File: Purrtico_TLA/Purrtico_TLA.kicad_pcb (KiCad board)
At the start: 2 copper layers, 100 x 50 mm, 67 parts, among them J1 XLR3, J3 Conn_01x02, J4 XLR3, J5 Conn_01x02, J7 Conn_02x05_Odd_Even, U1 OPA1679, U2 OPA1679

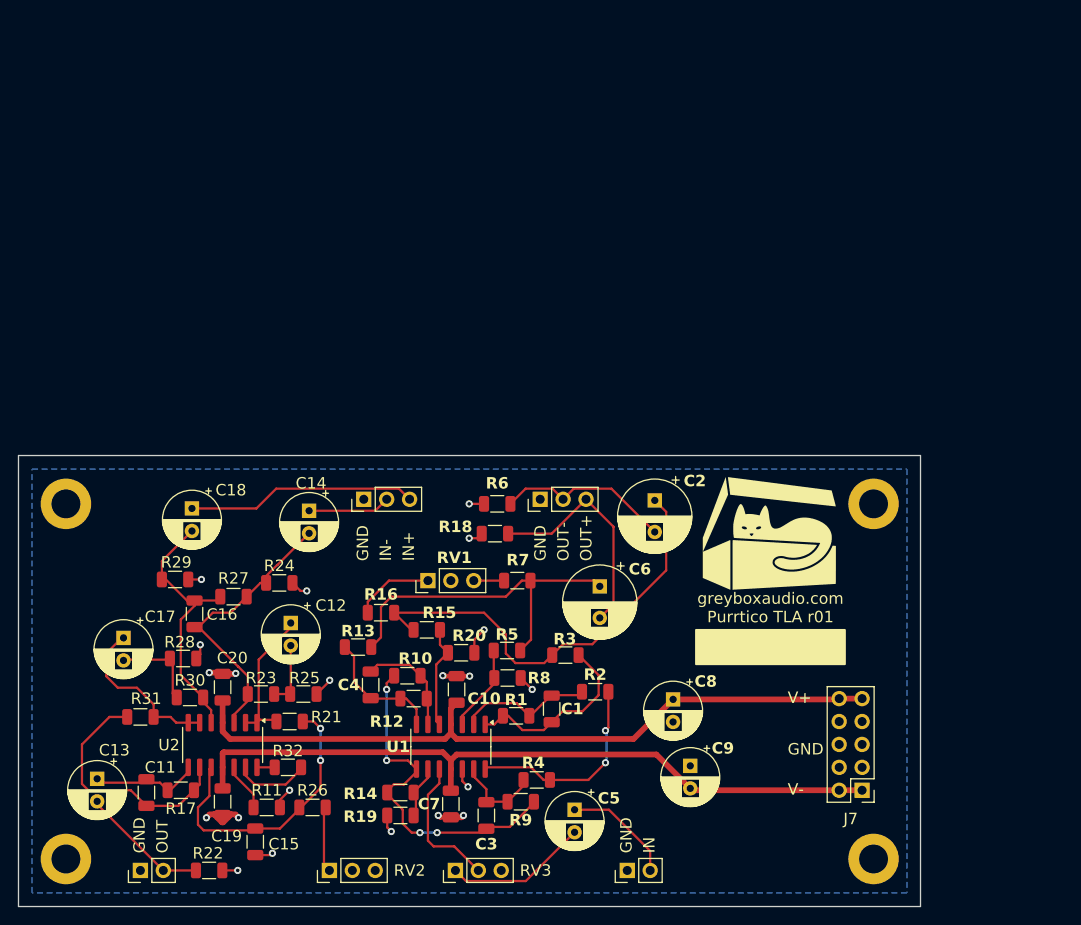
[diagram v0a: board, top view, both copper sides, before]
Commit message: update pcb
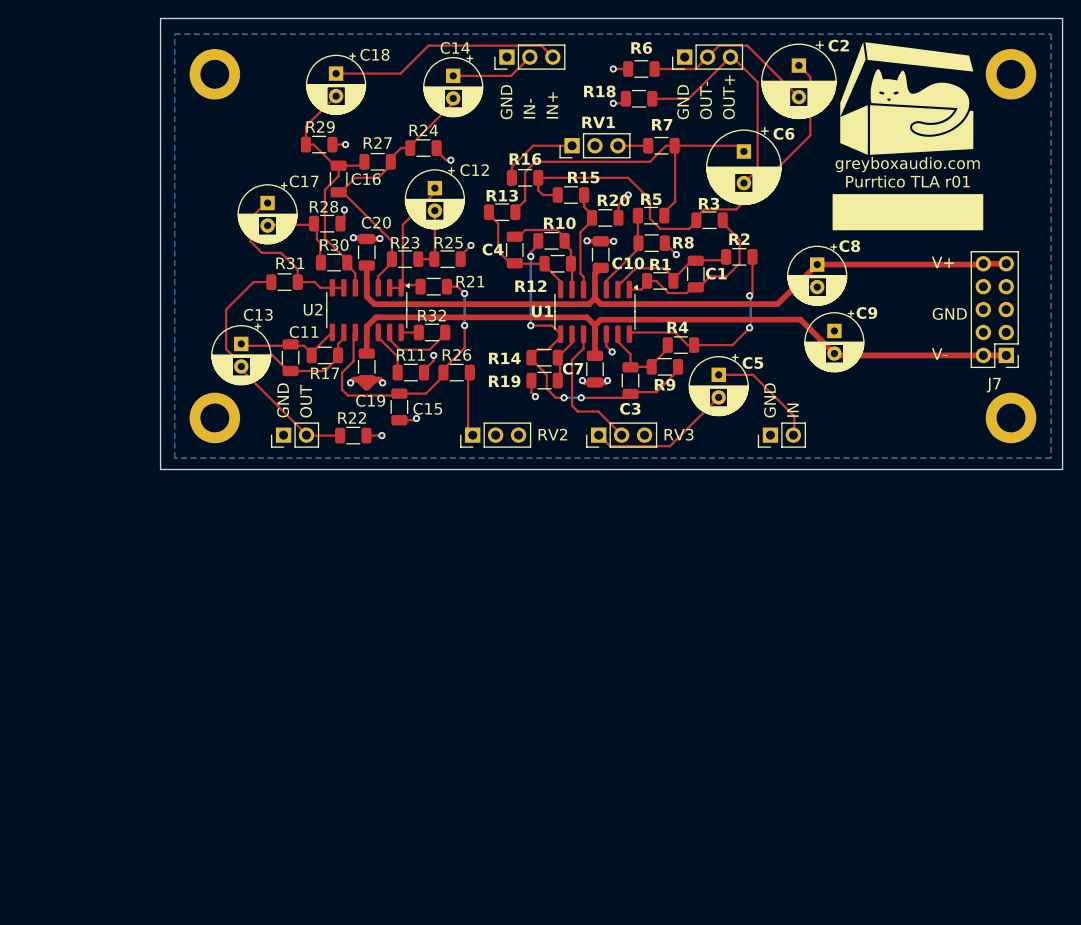
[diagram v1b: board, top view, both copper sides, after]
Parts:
- moved H3 51.6 mm to (64.8, 76.8)
- moved J1 51.6 mm to (116.9, 36.8)
- moved J4 51.5 mm to (97.2, 36.8)
- moved H4 51.2 mm to (153.0, 76.8)
- moved RV2 50.8 mm to (93.4, 78.7)
- moved RV3 50.8 mm to (107.3, 78.7)
- moved J3 50.8 mm to (126.4, 78.7)
- moved J5 50.8 mm to (72.4, 78.7)
- moved C11 50.8 mm to (73.2, 70.2)
- moved C13 50.8 mm to (67.7, 68.6)
- moved C15 50.8 mm to (85.2, 75.6)
- moved C16 50.8 mm to (78.5, 50.3)
- moved C20 50.8 mm to (81.6, 58.5)
- moved C5 50.8 mm to (120.6, 72.1)
- moved C6 50.8 mm to (123.4, 47.3)
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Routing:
- net Net-(C1-Pad2): track 20.6 -> 18.9 mm
- net Net-(U2A-+): track 29.9 -> 28.4 mm
- net Net-(C6-Pad2): track 25.3 -> 26.7 mm
- net Net-(U1A--): track 14.4 -> 13.0 mm
- net Net-(U2C--): track 27.6 -> 26.6 mm
- net Net-(C4-Pad2): track 14.0 -> 13.1 mm
- net Net-(U1B--): track 11.9 -> 10.9 mm
- net Net-(U2D--): track 8.46 -> 7.60 mm
- net Net-(U2B-+): track 28.8 -> 28.1 mm
- net GND: track 40.3 -> 39.6 mm
- net Net-(C2-Pad1): track 48.9 -> 49.6 mm
- net Net-(U2C-+): track 31.1 -> 30.4 mm
- net Net-(C3-Pad1): track 37.3 -> 36.6 mm
- net Net-(U1B-+): track 11.5 -> 10.9 mm
- net Net-(C6-Pad1): track 37.9 -> 37.3 mm
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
